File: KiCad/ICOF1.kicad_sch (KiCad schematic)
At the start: 40 parts, among them J1 USB C Connector, J2 JTAG_TC2030, SW1 Boot, U1 XC6206, U2 USBLC6-2SC6, U3 RP2040, U4 W25Q128JVS, Y1 12MHz

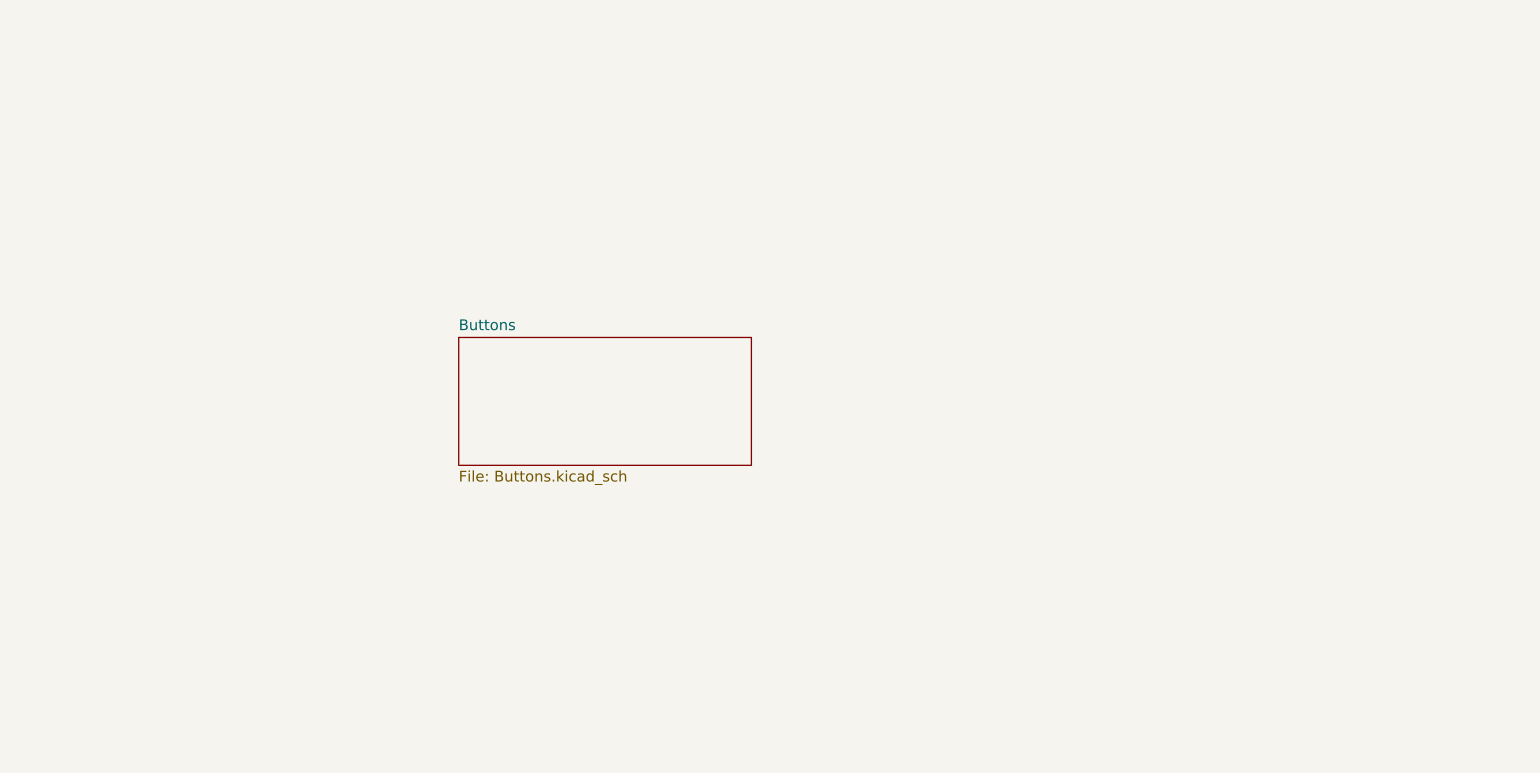
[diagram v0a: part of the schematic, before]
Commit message: v1.4
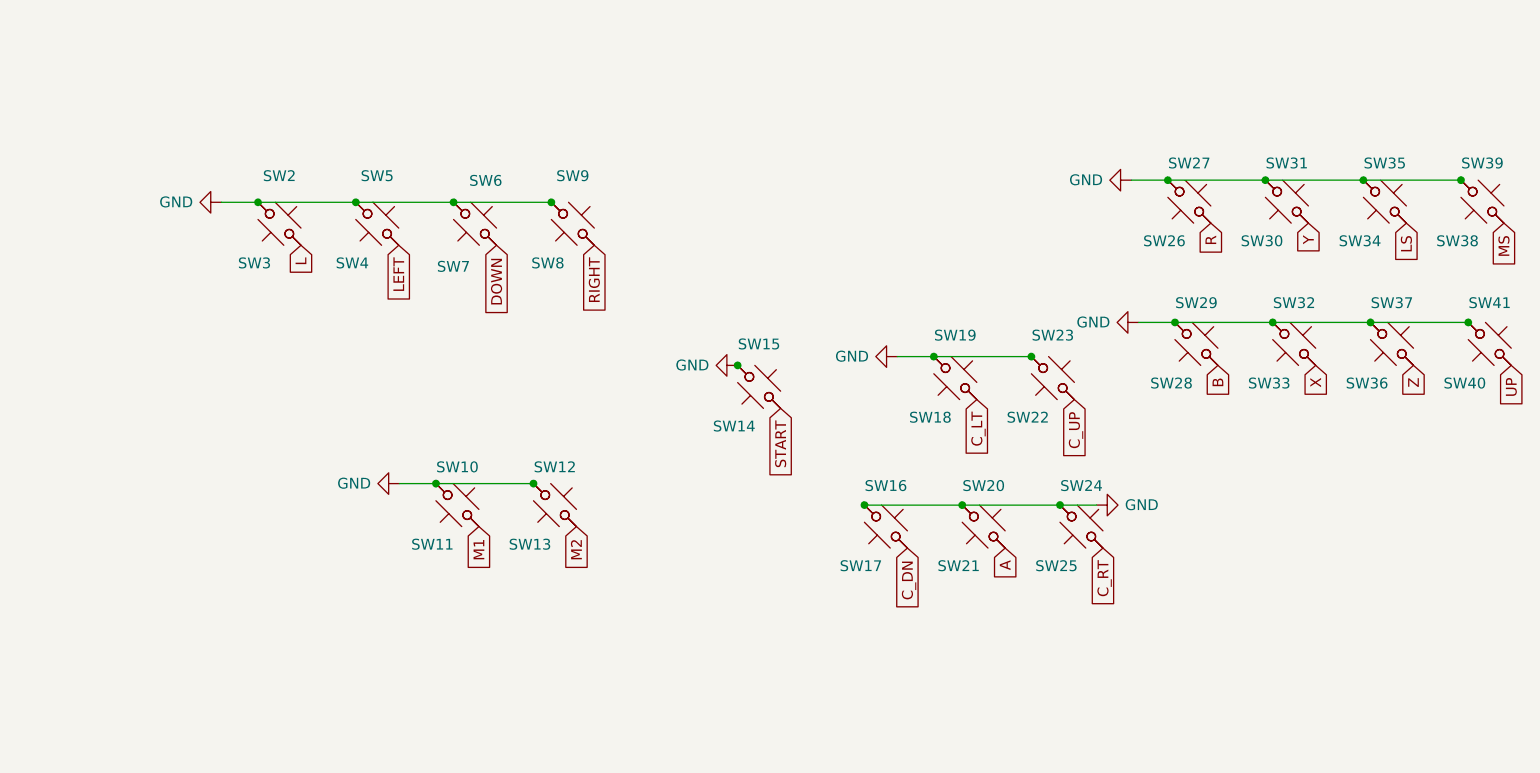
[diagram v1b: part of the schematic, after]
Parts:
- added SW10, SW12, SW15, SW16, SW19, SW2, SW20, SW23, SW24, SW27, SW29, SW31, SW32, SW35, SW37, SW39, SW41, SW5, SW7, SW9: MX_SW_HS, marbastlib-mx:SW_MX_HS_1u, symbol marbastlib-mx:MX_SW_HS
- added SW11, SW13, SW14, SW17, SW18, SW21, SW22, SW25, SW26, SW28, SW3, SW30, SW33, SW34, SW36, SW38, SW4, SW40, SW6, SW8: MX_SW_solder, marbastlib-mx:SW_MX_1u, symbol marbastlib-mx:MX_SW_solder
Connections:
- net A: now also SW20.2, SW21.1
- net B: now also SW28.1, SW29.2
- net C_DN: now also SW16.2, SW17.1
- net C_LT: now also SW18.1, SW19.2
- net C_RT: now also SW24.2, SW25.1
- net C_UP: now also SW22.1, SW23.2
- net DOWN: now also SW6.2, SW7.1
- net GND: now also SW10.1, SW11.2, SW12.1, SW13.2, SW14.2, SW15.1, SW16.1, SW17.2, SW18.2, SW19.1, SW2.1, SW20.1, SW21.2, SW22.2, SW23.1, SW24.1, SW25.2, SW26.2, SW27.1, SW28.2, SW29.1, SW3.2, SW30.2, SW31.1, SW32.1, SW33.2, SW34.2, SW35.1, SW36.2, SW37.1, SW38.2, SW39.1, SW4.2, SW40.2, SW41.1, SW5.1, SW6.1, SW7.2, SW8.2, SW9.1
- net L: now also SW2.2, SW3.1
- net LEFT: now also SW4.1, SW5.2
- net LS: now also SW34.1, SW35.2
- net M1: now also SW10.2, SW11.1
- net M2: now also SW12.2, SW13.1
- net MS: now also SW38.1, SW39.2
- net R: now also SW26.1, SW27.2
- net RIGHT: now also SW8.1, SW9.2
- net START: now also SW14.1, SW15.2
- net UP: now also SW40.1, SW41.2
- net X: now also SW32.2, SW33.1
- net Y: now also SW30.1, SW31.2
- net Z: now also SW36.1, SW37.2
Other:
- removed sheet Buttons

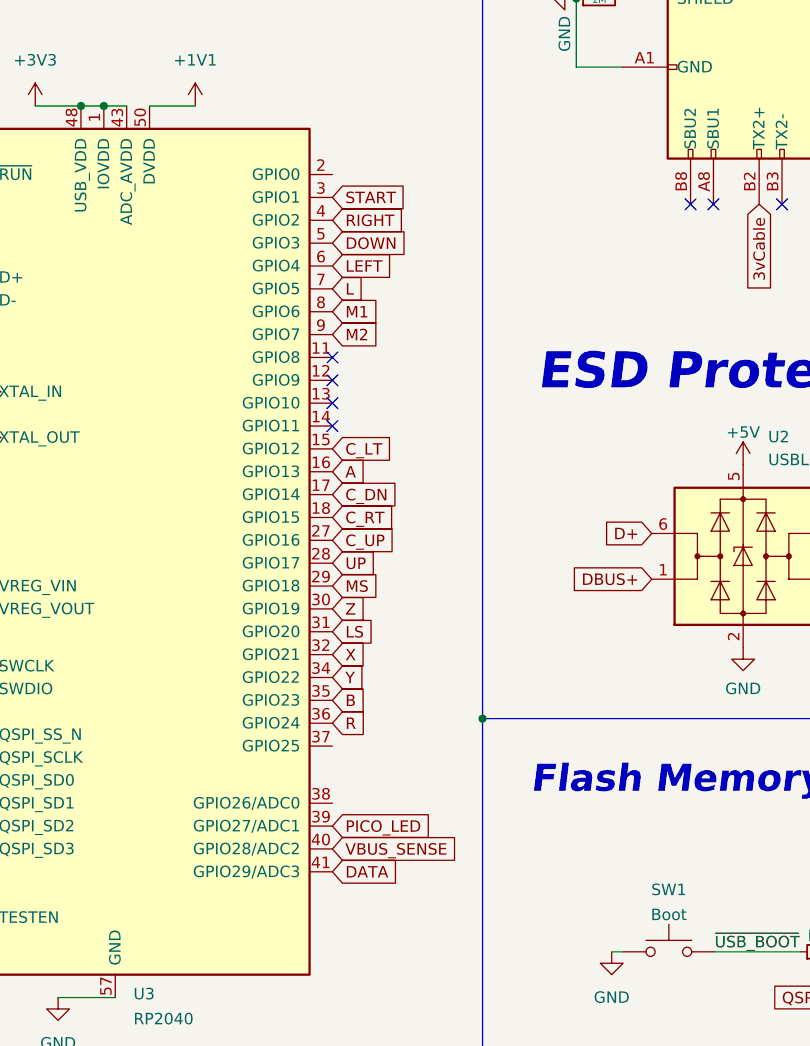
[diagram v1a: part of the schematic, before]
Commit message: final final v1.2
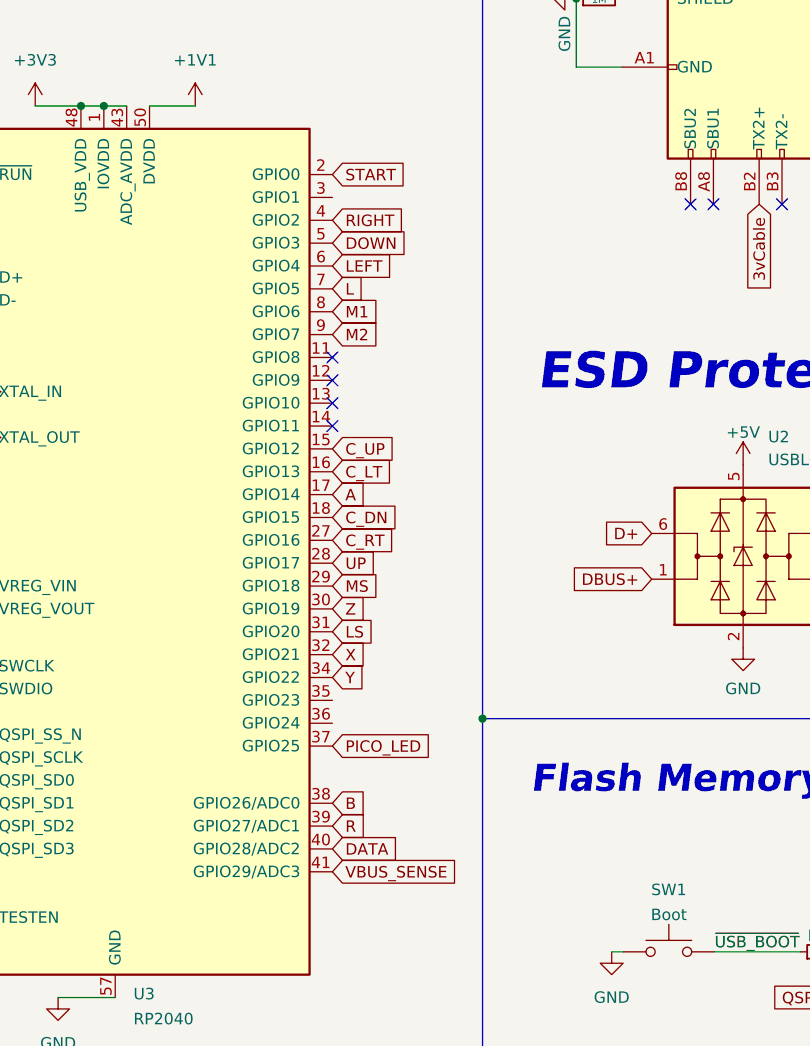
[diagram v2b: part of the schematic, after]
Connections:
- net A: now also U3.17 (GPIO14); no longer U3.16 (GPIO13)
- net B: now also U3.38 (GPIO26/ADC0); no longer U3.35 (GPIO23)
- net C_DN: now also U3.18 (GPIO15); no longer U3.17 (GPIO14)
- net C_LT: now also U3.16 (GPIO13); no longer U3.15 (GPIO12)
- net C_RT: now also U3.27 (GPIO16); no longer U3.18 (GPIO15)
- net C_UP: now also U3.15 (GPIO12); no longer U3.27 (GPIO16)
- net DATA: now also U3.40 (GPIO28/ADC2); no longer U3.41 (GPIO29/ADC3)
- net PICO_LED: now also U3.37 (GPIO25); no longer U3.39 (GPIO27/ADC1)
- net R: now also U3.39 (GPIO27/ADC1); no longer U3.36 (GPIO24)
- net START: now also U3.2 (GPIO0); no longer U3.3 (GPIO1)
- net VBUS_SENSE: now also U3.41 (GPIO29/ADC3); no longer U3.40 (GPIO28/ADC2)
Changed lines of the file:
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@@
+    )
+  )
+  (global_label "VBUS_SENSE" (shape input) (at 71.9648 125.984 0) (fields_autoplaced)
+    (effects (font (size 1.27 1.27)) (justify left))
+    (property "Intersheetrefs" "${INTERSHEET_REFS}" (at 86.7843 125.984 0)
+      (effects (font (size 1.27 1.27)) (justify left) hide)
     )
   )
@@
     )
   )
+  (global_label "PICO_LED" (shape input) (at 71.9648 112.014 0) (fields_autoplaced)
+    (effects (font (size 1.27 1.27)) (justify left))
+    (property "Intersheetrefs" "${INTERSHEET_REFS}" (at 83.7606 112.014 0)
+      (effects (font (size 1.27 1.27)) (justify left) hide)
+    )
+  )
   (global_label "D+" (shape input) (at 21.114 59.944 180) (fields_autoplaced)
     (effects (font (size 1.27 1.27)) (justify right))
@@
     )
   )
+  (global_label "DATA" (shape input) (at 71.9648 123.444 0) (fields_autoplaced)
+    (effects (font (size 1.27 1.27)) (justify left))
+    (property "Intersheetrefs" "${INTERSHEET_REFS}" (at 78.7927 123.3646 0)
+      (effects (font (size 1.27 1.27)) (justify left) hide)
+    )
+  )
   (global_label "RIGHT" (shape input) (at 258.6482 133.1214 270) (fields_autoplaced)
     (effects (font (size 1.27 1.27)) (justify right))
@@
     )
   )
-  (global_label "START" (shape input) (at 71.9648 51.054 0) (fields_autoplaced)
-    (effects (font (size 1.27 1.27)) (justify left))
-    (property "Intersheetrefs" "${INTERSHEET_REFS}" (at 80.3739 51.054 0)
-      (effects (font (size 1.27 1.27)) (justify left) hide)
-    )
-  )
   (global_label "SD3" (shape input) (at 156.972 142.494 0) (fields_autoplaced)
     (effects (font (size 1.27 1.27)) (justify left))
@@
     )
   )
-  (global_label "R" (shape input) (at 71.9648 109.474 0) (fields_autoplaced)
-    (effects (font (size 1.27 1.27)) (justify left))
-    (property "Intersheetrefs" "${INTERSHEET_REFS}" (at 76.1406 109.474 0)
-      (effects (font (size 1.27 1.27)) (justify left) hide)
-    )
-  )
   (global_label "CS" (shape input) (at 130.302 134.874 90) (fields_autoplaced)
     (effects (font (size 1.27 1.27)) (justify left))
@@
     )
   )
+  (global_label "R" (shape input) (at 71.9648 120.904 0) (fields_autoplaced)
+    (effects (font (size 1.27 1.27)) (justify left))
+    (property "Intersheetrefs" "${INTERSHEET_REFS}" (at 76.1406 120.904 0)
+      (effects (font (size 1.27 1.27)) (justify left) hide)
+    )
+  )
   (global_label "SD3" (shape input) (at 31.3248 123.444 180) (fields_autoplaced)
     (effects (font (size 1.27 1.27)) (justify right))
@@
     )
   )
-  (global_label "PICO_LED" (shape input) (at 71.9648 120.904 0) (fields_autoplaced)
-    (effects (font (size 1.27 1.27)) (justify left))
-    (property "Intersheetrefs" "${INTERSHEET_REFS}" (at 83.7606 120.904 0)
-      (effects (font (size 1.27 1.27)) (justify left) hide)
-    )
-  )
-  (global_label "C_LT" (shape input) (at 71.9648 78.994 0) (fields_autoplaced)
-    (effects (font (size 1.27 1.27)) (justify left))
-    (property "Intersheetrefs" "${INTERSHEET_REFS}" (at 79.1039 78.994 0)
-      (effects (font (size 1.27 1.27)) (justify left) hide)
-    )
-  )
-  (global_label "B" (shape input) (at 71.9648 106.934 0) (fields_autoplaced)
-    (effects (font (size 1.27 1.27)) (justify left))
-    (property "Intersheetrefs" "${INTERSHEET_REFS}" (at 76.1406 106.934 0)
+  (global_label "C_UP" (shape input) (at 71.9648 78.994 0) (fields_autoplaced)
+    (effects (font (size 1.27 1.27)) (justify left))
+    (property "Intersheetrefs" "${INTERSHEET_REFS}" (at 79.7087 78.994 0)
       (effects (font (size 1.27 1.27)) (justify left) hide)
     )
@@
     )
   )
-  (global_label "A" (shape input) (at 71.9648 81.534 0) (fields_autoplaced)
-    (effects (font (size 1.27 1.27)) (justify left))
-    (property "Intersheetrefs" "${INTERSHEET_REFS}" (at 75.4665 81.4546 0)
+  (global_label "C_LT" (shape input) (at 71.9648 81.534 0) (fields_autoplaced)
+    (effects (font (size 1.27 1.27)) (justify left))
+    (property "Intersheetrefs" "${INTERSHEET_REFS}" (at 79.1039 81.534 0)
       (effects (font (size 1.27 1.27)) (justify left) hide)
     )
@@
     )
   )
-  (global_label "C_DN" (shape input) (at 71.9648 84.074 0) (fields_autoplaced)
-    (effects (font (size 1.27 1.27)) (justify left))
-    (property "Intersheetrefs" "${INTERSHEET_REFS}" (at 79.7087 84.074 0)
+  (global_label "A" (shape input) (at 71.9648 84.074 0) (fields_autoplaced)
+    (effects (font (size 1.27 1.27)) (justify left))
+    (property "Intersheetrefs" "${INTERSHEET_REFS}" (at 75.9592 84.074 0)
       (effects (font (size 1.27 1.27)) (justify left) hide)
     )
@@
     )
   )
-  (global_label "DATA" (shape input) (at 71.9648 125.984 0) (fields_autoplaced)
-    (effects (font (size 1.27 1.27)) (justify left))
-    (property "Intersheetrefs" "${INTERSHEET_REFS}" (at 78.7927 125.9046 0)
-      (effects (font (size 1.27 1.27)) (justify left) hide)
-    )
-  )
-  (global_label "C_RT" (shape input) (at 71.9648 86.614 0) (fields_autoplaced)
-    (effects (font (size 1.27 1.27)) (justify left))
-    (property "Intersheetrefs" "${INTERSHEET_REFS}" (at 78.8531 86.5346 0)
+  (global_label "B" (shape input) (at 71.9648 118.364 0) (fields_autoplaced)
+    (effects (font (size 1.27 1.27)) (justify left))
+    (property "Intersheetrefs" "${INTERSHEET_REFS}" (at 76.1406 118.364 0)
+      (effects (font (size 1.27 1.27)) (justify left) hide)
+    )
+  )
+  (global_label "C_DN" (shape input) (at 71.9648 86.614 0) (fields_autoplaced)
+    (effects (font (size 1.27 1.27)) (justify left))
+    (property "Intersheetrefs" "${INTERSHEET_REFS}" (at 79.7087 86.614 0)
+      (effects (font (size 1.27 1.27)) (justify left) hide)
+    )
+  )
+  (global_label "START" (shape input) (at 71.9648 48.514 0) (fields_autoplaced)
+    (effects (font (size 1.27 1.27)) (justify left))
+    (property "Intersheetrefs" "${INTERSHEET_REFS}" (at 80.3739 48.514 0)
       (effects (font (size 1.27 1.27)) (justify left) hide)
     )
@@
     )
   )
-  (global_label "C_UP" (shape input) (at 71.9648 89.154 0) (fields_autoplaced)
-    (effects (font (size 1.27 1.27)) (justify left))
-    (property "Intersheetrefs" "${INTERSHEET_REFS}" (at 79.216 89.0746 0)
+  (global_label "C_RT" (shape input) (at 71.9648 89.154 0) (fields_autoplaced)
+    (effects (font (size 1.27 1.27)) (justify left))
+    (property "Intersheetrefs" "${INTERSHEET_REFS}" (at 79.3458 89.154 0)
       (effects (font (size 1.27 1.27)) (justify left) hide)
     )
@@
       (effects (font (size 1.27 1.27)) (justify left) hide)
     )
-  )
-  (global_label "VBUS_SENSE" (shape input) (at 71.9648 123.444 0) (fields_autoplaced)
-    (effects (font (size 1.27 1.27)) (justify left))
-    (property "Intersheetrefs" "${INTERSHEET_REFS}" (at 86.7843 123.444 0)
-      (effects (font (size 1.27 1.27)) (justify left) hide)
-    )
